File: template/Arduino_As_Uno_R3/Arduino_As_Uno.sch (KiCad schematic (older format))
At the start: 8 parts, among them P1 Power, P2 Analog, P3 Digital, P4 Digital, P5 CONN_1, P6 CONN_1, P7 CONN_1, P8 CONN_1

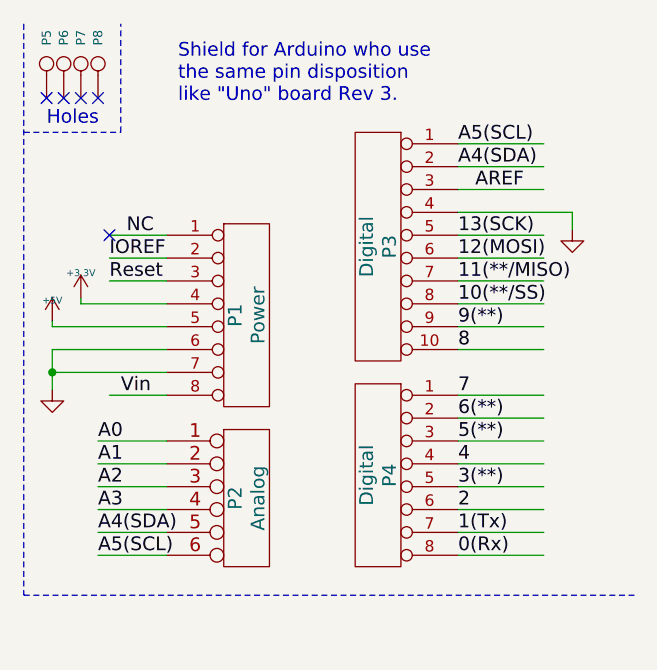
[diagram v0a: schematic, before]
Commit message: Correction schématics
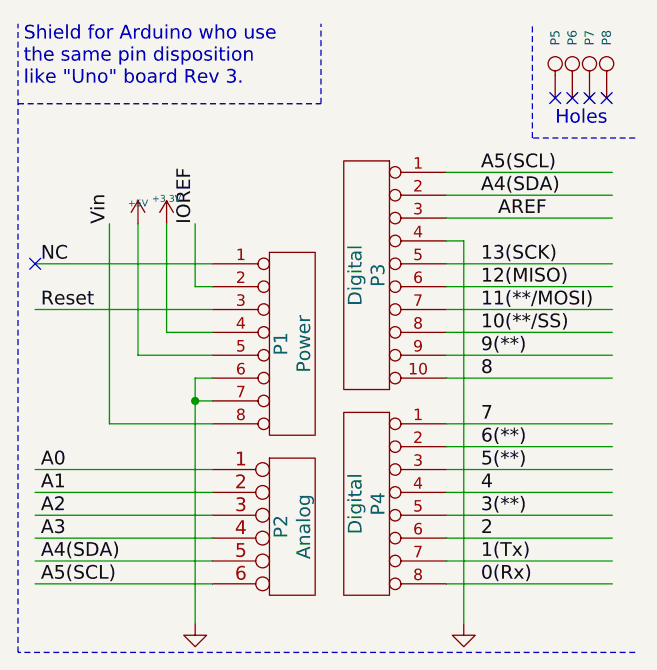
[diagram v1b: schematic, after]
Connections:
- net labels added: 11(**/MOSI), 12(MISO)
- net labels removed: 11(**/MISO), 12(MOSI)
- wire segments 36 -> 38
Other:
- moved on the sheet: P1, P2, P3, P4, P5, P6, P7, P8
